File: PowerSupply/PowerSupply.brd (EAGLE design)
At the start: 36.6 x 29.8 mm, 19 parts, among them Q2 DMMT5401, Q3 DMG2305UX

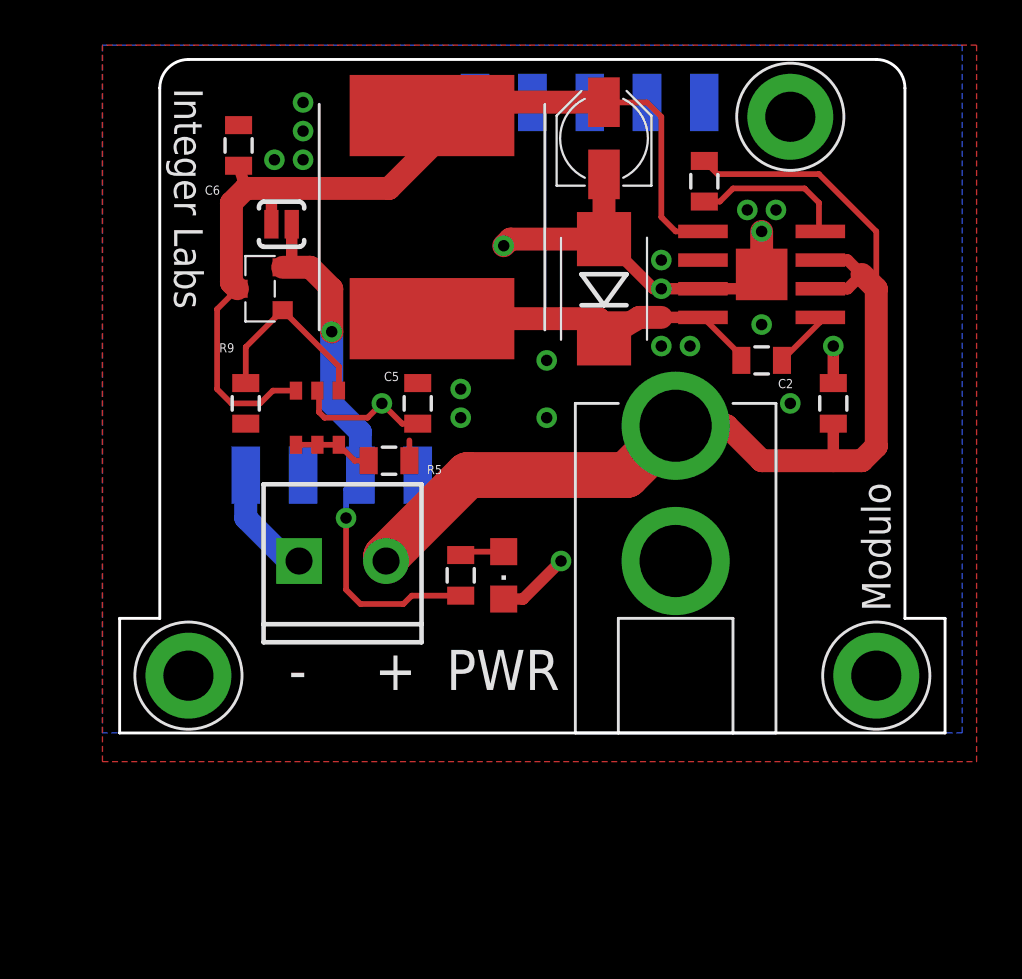
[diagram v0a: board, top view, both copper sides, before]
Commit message: various minor changes
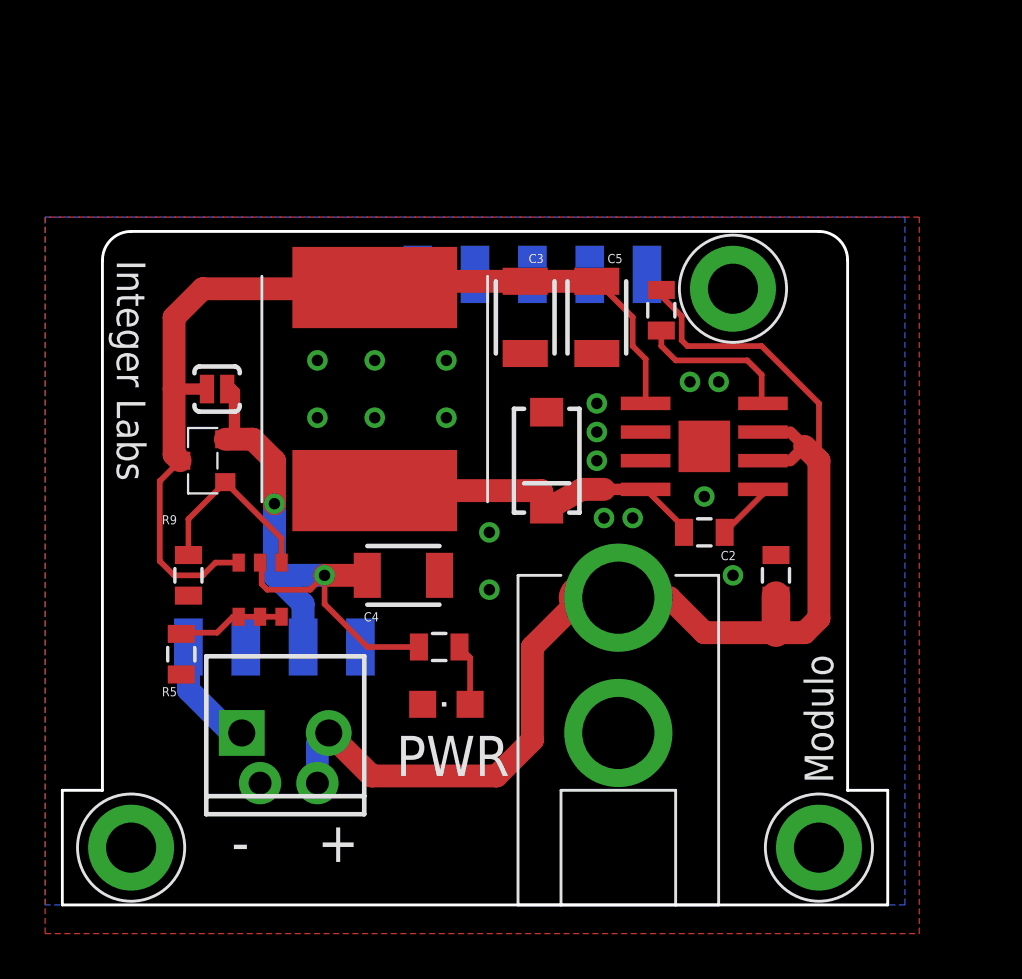
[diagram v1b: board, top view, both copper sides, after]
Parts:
- removed C6: .47uF, SparkFun-Capacitors:0805
- added C3: 47uF, SparkFun-Capacitors:1210
- added JP1: M021X02_NO_SILK, SparkFun-Connectors:1X02_NO_SILK
- C4: value (none) -> 47uF; device adafruit:PANASONIC_B -> SparkFun-Capacitors:1210
- C5: device SparkFun-Capacitors:0805 -> SparkFun-Capacitors:1210
- D1: value ssb43L -> ssa33l; device SparkFun-DiscreteSemi:SMB-DIODE -> SparkFun-DiscreteSemi:SMA-DIODE
- L1: value 4.7uH -> 15uH
- moved C4 21.3 mm to (14.6, 14.6), turned to 0 degrees
- moved R5 12.6 mm to (4.76, 11.1), turned to 90 degrees
- moved C5 8.80 mm to (23.2, 26.0), turned to 270 degrees
- moved C1 8.03 mm to (31.1, 14.6)
- moved D1 8.03 mm to (21.0, 19.7), turned to 270 degrees
- moved JP5 8.03 mm to (7.62, 7.62)
- moved Q3 8.03 mm to (5.71, 19.7)
- moved R9 8.03 mm to (5.08, 14.6)
- moved U$21 8.03 mm to (24.1, 7.62)
- moved U$4 8.03 mm to (0.00, 0.00)
- moved L1 8.03 mm to (13.3, 22.9)
- moved Q2 8.03 mm to (8.26, 14.0)
- moved U$3 8.03 mm to (27.9, 20.3)
- moved C2 8.03 mm to (27.9, 16.5)
- moved SJ1 7.84 mm to (6.35, 22.9)
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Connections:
- net GND: now also C3.2, C4.2, JP1.1; no longer C4.-, C6.2
- net VCC: now also C4.1; no longer C5.1
- net VIN: now also JP1.2
- net VREG: now also C3.1, C5.1; no longer C4.+, C6.1
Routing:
- net GND: track 28.7 -> 4.60 mm, vias 20 -> 17
- net VIN: track 50.4 -> 57.7 mm
- net VCC: track 30.4 -> 28.5 mm, vias 3 -> 2
- net N$14: track 3.52 -> 4.76 mm
- net N$8: track 1.97 -> 2.73 mm
- net VREG: track 43.8 -> 43.2 mm

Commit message: Checkpointing PCB designs
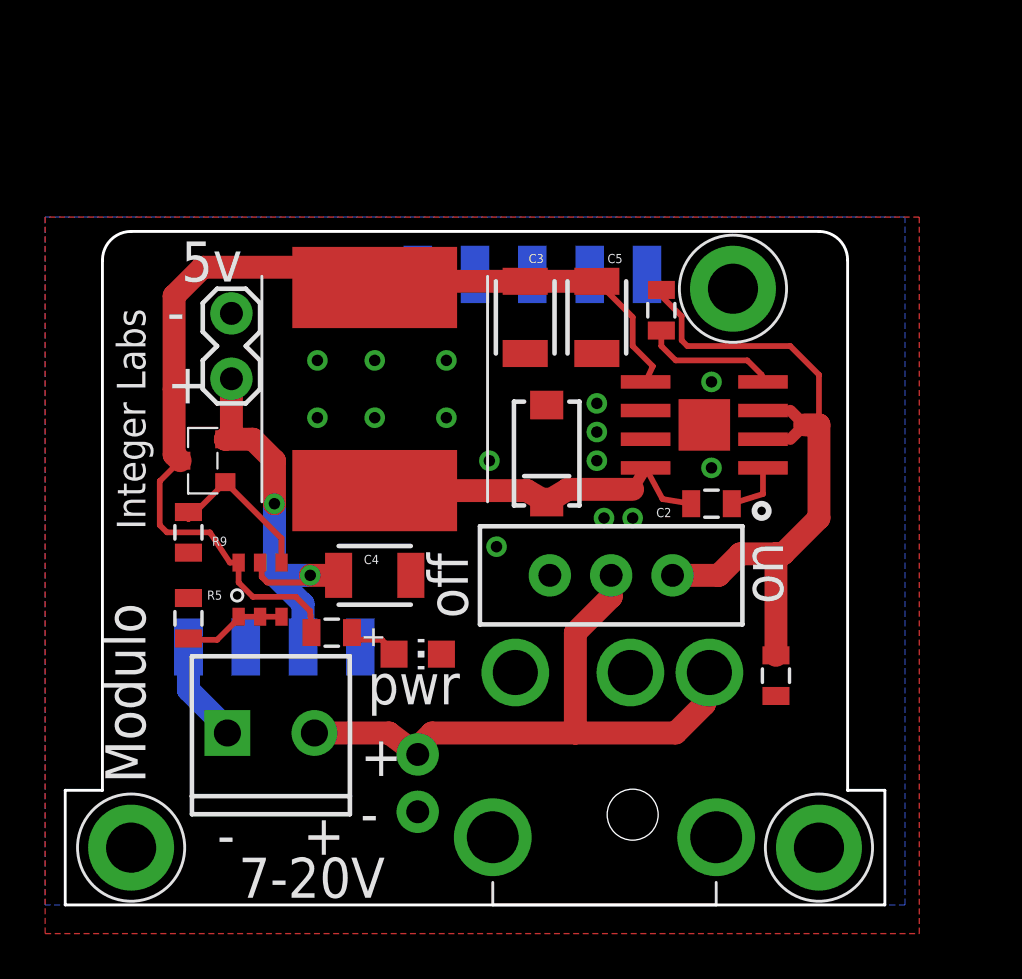
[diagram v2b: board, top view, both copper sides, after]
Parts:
- removed SJ1: SOLDERJUMPERNO, SparkFun-Passives:SJ_2S-NO
- added JP2: M02LOCK, SparkFun-Connectors:1X02_LOCK
- added S2: (no value), SparkFun-Electromechanical:SWITCH-SPDT_LOCK.007S
- LED1: device led:CHIPLED_0805 -> adafruit:CHIP-LED0805
- U$21: value DC-JACK -> DC-JACKLOWPRO; device IntegerLabs:DC-POWER-JACK -> IntegerLabs:DC-POWER-JACK-LOWPRO
- moved U$21 7.65 mm to (24.8, 0.00)
- moved JP1 7.10 mm to (15.2, 4.13), turned to 90 degrees
- moved R2 4.80 mm to (11.4, 12.1)
- moved C1 4.45 mm to (31.1, 10.2), turned to 270 degrees
- moved LED1 2.56 mm to (15.2, 11.1), turned to 270 degrees
- moved R9 1.91 mm to (5.08, 16.5)
- moved R5 1.62 mm to (5.08, 12.7), turned to 270 degrees
- moved C2 1.31 mm to (28.3, 17.8)
- moved C4 1.27 mm to (13.3, 14.6)
- moved U$3 0.95 mm to (27.9, 21.3)
- moved JP5 0.63 mm to (6.99, 7.62)
- moved D1 0.32 mm to (21.0, 20.0)
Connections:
- new net N$2: JP1.2, JP5.2, S2.2, U$21.1
- net GND: now also JP2.1, U$21.2; no longer U$21.P2
- net VCC: now also JP2.2; no longer R2.2, SJ1.2
- net VIN: now also S2.3; no longer JP1.2, JP5.2, U$21.P1
- net VREG: now also R2.2; no longer SJ1.1
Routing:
- net N$2: track 0.00 -> 27.8 mm
- net VIN: track 57.7 -> 32.6 mm
- net VCC: track 28.5 -> 20.7 mm
- net VREG: track 43.2 -> 47.4 mm
- net N$16: track 8.50 -> 7.22 mm
- net N$6: track 6.95 -> 6.00 mm
- net GND: vias 17 -> 15
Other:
- board size 36.6 x 29.8 mm -> 36.3 x 29.8 mm
- board text added: "5v"
- board text added: "7-20V"
- board text added: "off"
- board text added: "on"
- board text added: "pwr"
- board text removed: "PWR"
